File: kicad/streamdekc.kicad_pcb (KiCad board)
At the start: 2 copper layers, 26 parts, among them IC1 74HC4051P, IC2 74HC4051P, SW1 SW_DIP_x01, SW2 SW_DIP_x01, SW3 SW_DIP_x01, SW4 SW_DIP_x01, SW5 SW_DIP_x01, SW6 SW_DIP_x01, SW7 SW_DIP_x01, SW8 SW_DIP_x01, U1_1 QT_PY_L, U1_2 QT_PY_R, U2_1 VOLTAGE_TRANSLATOR_L, U2_2 VOLTAGE_TRANSLATOR_R

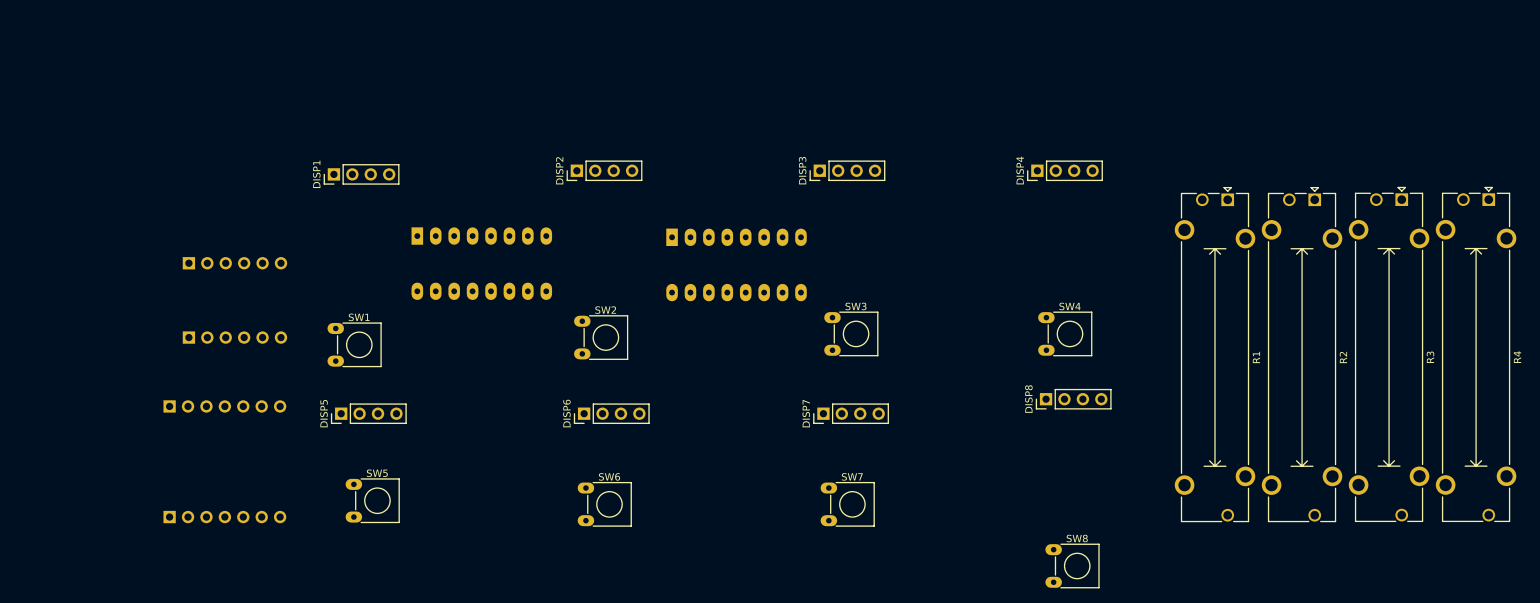
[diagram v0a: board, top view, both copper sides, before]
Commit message: Initial pcb design
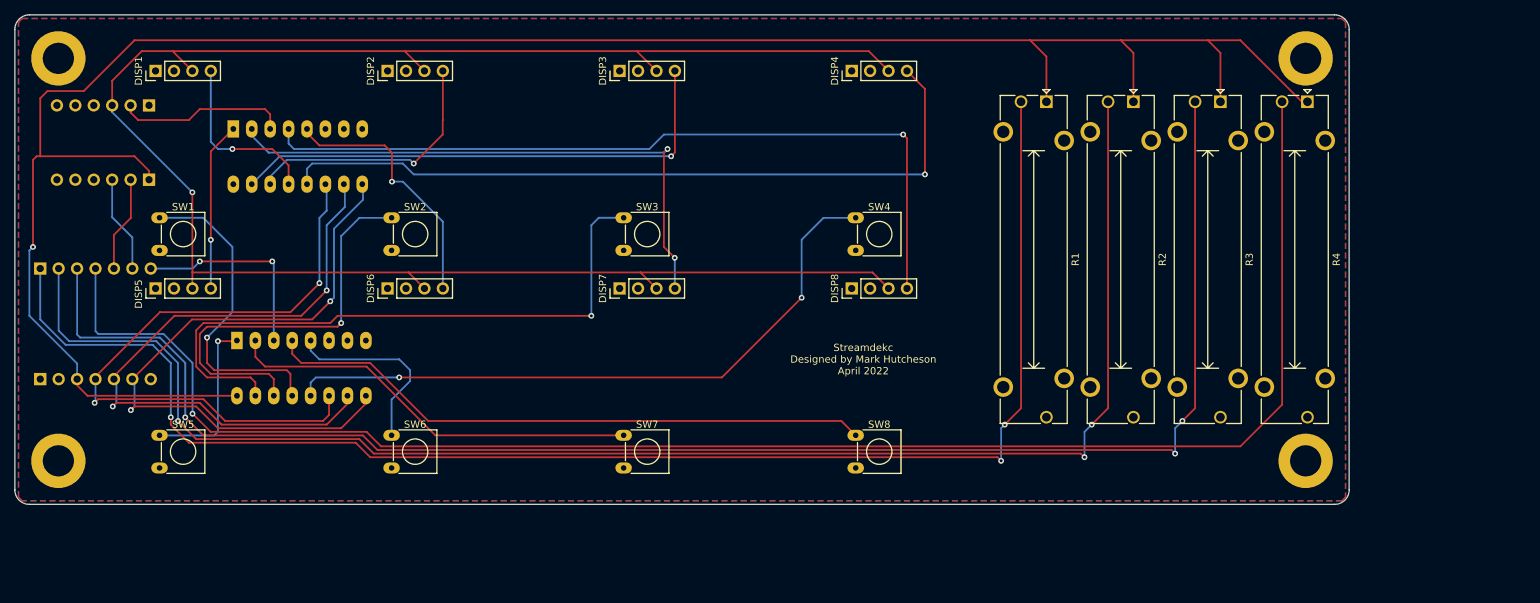
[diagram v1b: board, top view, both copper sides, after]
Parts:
- added REF**: MountingHole_4.3mm_M4_DIN965_Pad, MountingHole:MountingHole_4.3mm_M4_DIN965_Pad, F.Cu at (67.0, 123.5)
- added REF**: MountingHole_4.3mm_M4_DIN965_Pad, MountingHole:MountingHole_4.3mm_M4_DIN965_Pad, F.Cu at (239.0, 68.0)
- added REF**: MountingHole_4.3mm_M4_DIN965_Pad, MountingHole:MountingHole_4.3mm_M4_DIN965_Pad, F.Cu at (67.0, 68.0)
- added REF**: MountingHole_4.3mm_M4_DIN965_Pad, MountingHole:MountingHole_4.3mm_M4_DIN965_Pad, F.Cu at (239.0, 123.5)
- moved IC2 61.7 mm to (91.6, 106.9)
- moved DISP7 33.0 mm to (144.4, 99.7)
- moved U2_2 32.5 mm to (79.5, 74.5), turned to 90 degrees
- moved DISP6 32.1 mm to (112.4, 99.7)
- moved SW3 31.9 mm to (148.2, 92.2)
- moved SW8 31.5 mm to (180.2, 122.2)
- moved DISP5 30.9 mm to (80.4, 99.7)
- moved DISP8 30.8 mm to (176.4, 99.7)
- moved DISP3 30.8 mm to (144.4, 69.7)
- moved SW2 29.9 mm to (116.2, 92.2)
- moved SW4 29.7 mm to (180.2, 92.2)
- moved DISP2 29.5 mm to (112.4, 69.7)
- moved IC1 29.4 mm to (91.1, 77.7)
- moved SW7 29.2 mm to (148.2, 122.2)
- moved DISP4 29.1 mm to (176.4, 69.7)
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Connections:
- SW1 pad 1: unconnected-(SW1-Pad1) -> /SW1
- SW2 pad 1: unconnected-(SW2-Pad1) -> /SW2
- SW3 pad 1: unconnected-(SW3-Pad1) -> /SW3
- SW4 pad 1: unconnected-(SW4-Pad1) -> /SW4
- SW5 pad 1: unconnected-(SW5-Pad1) -> /SW5
- SW6 pad 1: unconnected-(SW6-Pad1) -> /SW6
- SW7 pad 1: unconnected-(SW7-Pad1) -> /SW7
- SW8 pad 1: unconnected-(SW8-Pad1) -> /SW8
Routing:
- net /3V3: track 0.00 -> 292.3 mm, vias 0 -> 1
- net /SCL_5V: track 0.00 -> 257.9 mm, vias 0 -> 1
- net /A3: track 0.00 -> 227.1 mm, vias 0 -> 1
- net /A2: track 0.00 -> 221.4 mm, vias 0 -> 3
- net /A1: track 0.00 -> 212.3 mm, vias 0 -> 3
- net /A0: track 0.00 -> 203.2 mm, vias 0 -> 3
- net /DISP_8_SDA: track 0.00 -> 109.4 mm, vias 0 -> 1
- net /DISP_4_SDA: track 0.00 -> 103.6 mm, vias 0 -> 1
- net /SW4: track 0.00 -> 91.1 mm, vias 0 -> 2
- net /D10: track 0.00 -> 90.8 mm, vias 0 -> 2
- net /D8: track 0.00 -> 90.7 mm, vias 0 -> 2
- net /D9: track 0.00 -> 90.6 mm, vias 0 -> 2
- net /SW3: track 0.00 -> 88.6 mm, vias 0 -> 1
- net /SW8: track 0.00 -> 84.2 mm
- net /DISP_7_SDA: track 0.00 -> 79.5 mm, vias 0 -> 2
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- added copper zone on F.Cu, net /5V
- added copper zone on B.Cu, net /GND
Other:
- board outline added: 184 x 67.5 mm
- board text added: "Order of Assembly: 1. Switches 2. ICs 3. Power Converter 4. Slide Potentiometers 5. Qt Py 6. Displays (Good luck)"
- board text added: "Streamdekc Designed by Mark Hutcheson April 2022"
